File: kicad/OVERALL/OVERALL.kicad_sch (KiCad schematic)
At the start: 0 parts

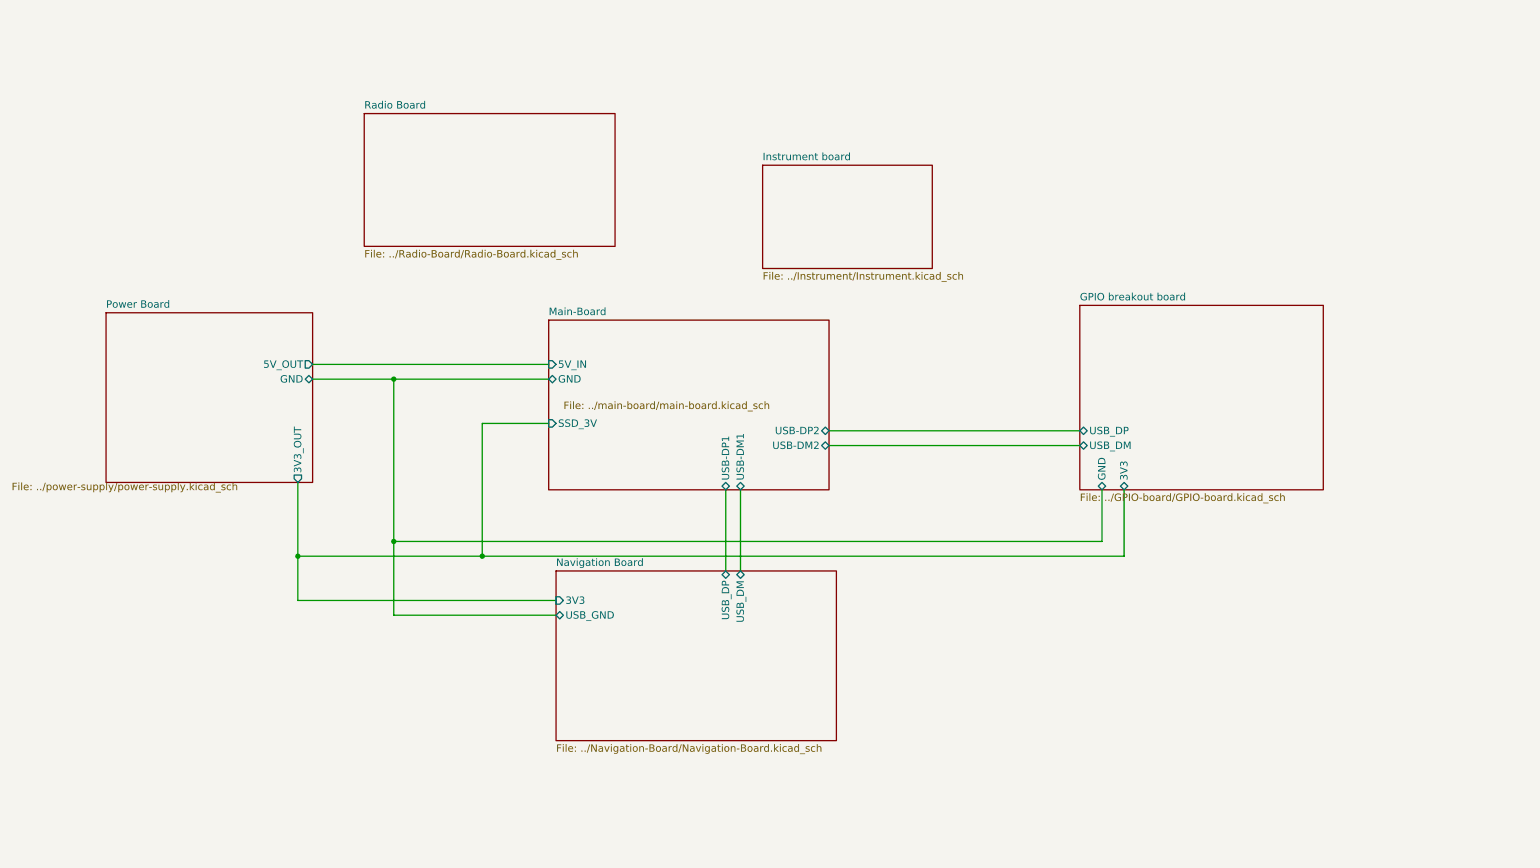
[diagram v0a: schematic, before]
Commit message: finally completed the schematic
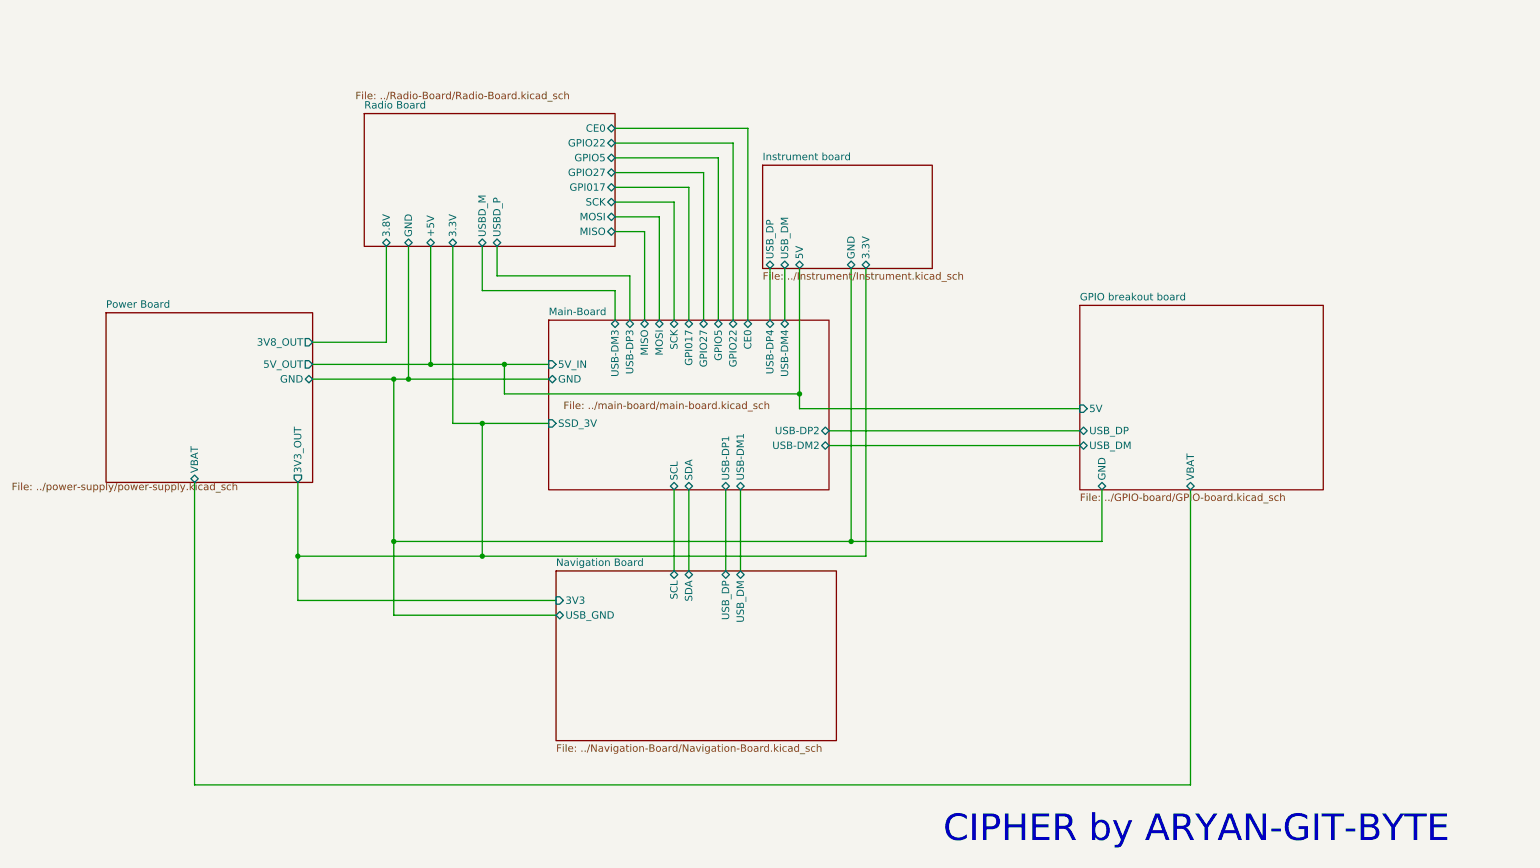
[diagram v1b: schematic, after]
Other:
- sheet GPIO breakout board ports: added 5V, VBAT; removed 3V3
- sheet Instrument board ports: added 3.3V, 5V, GND, USB_DM, USB_DP; removed none
- sheet Main-Board ports: added CE0, GPI017, GPIO22, GPIO27, GPIO5, MISO, MOSI, SCK, SCL, SDA, USB-DM3, USB-DM4, USB-DP3, USB-DP4; removed none
- sheet Navigation Board ports: added SCL, SDA; removed none
- sheet Power Board ports: added 3V8_OUT, VBAT; removed none
- sheet Radio Board ports: added +5V, 3.3V, 3.8V, CE0, GND, GPI017, GPIO22, GPIO27, GPIO5, MISO, MOSI, SCK, USBD_M, USBD_P; removed none
- note added: "CIPHER by ARYAN-GIT-BYTE"

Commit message: all data got corrupted bruhh. now , commiting whats left healthy
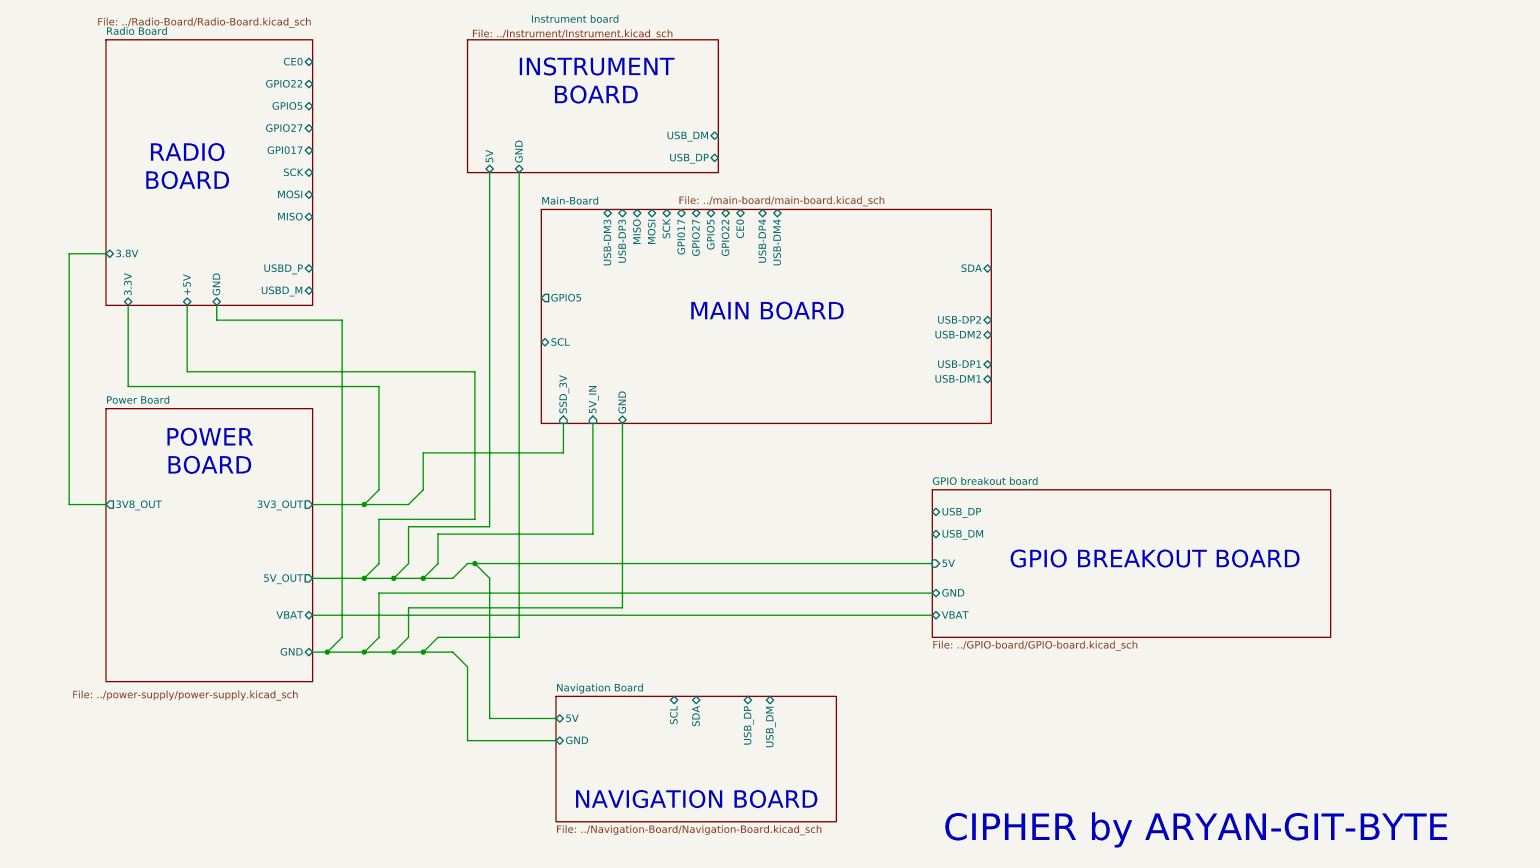
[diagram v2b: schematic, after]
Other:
- sheet Instrument board ports: added none; removed 3.3V
- sheet Navigation Board ports: added 5V, GND; removed 3V3, USB_GND
- note added: "GPIO BREAKOUT BOARD"
- note added: "INSTRUMENT BOARD"
- note added: "MAIN BOARD"
- note added: "NAVIGATION BOARD"
- note added: "POWER BOARD"
- note added: "RADIO BOARD"
